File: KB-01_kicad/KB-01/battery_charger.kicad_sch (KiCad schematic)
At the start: 37 parts, among them IC1 MAX17048G+T10, J12 Conn_01x01_Socket, J3 USB_C_Receptacle_USB2.0_14P, J4 Conn_01x02_Socket, J5 Conn_01x01_Socket, SW2 Power button, U1 BQ25895, U2 TS3USB30ERSWR, U3 TLV70430DBVR

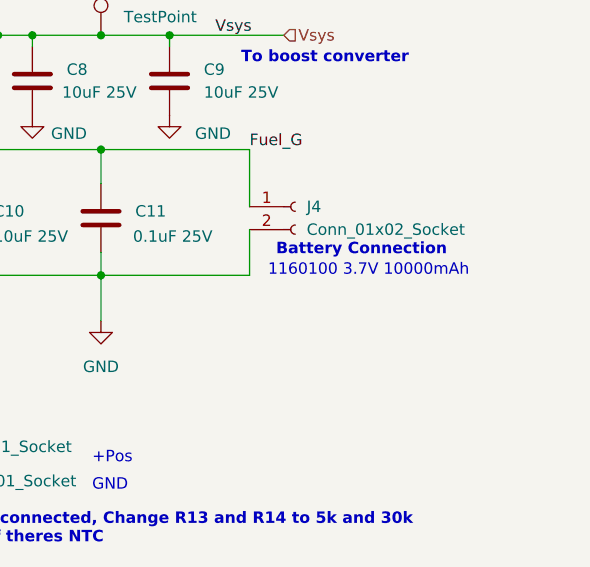
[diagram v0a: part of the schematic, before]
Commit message: all
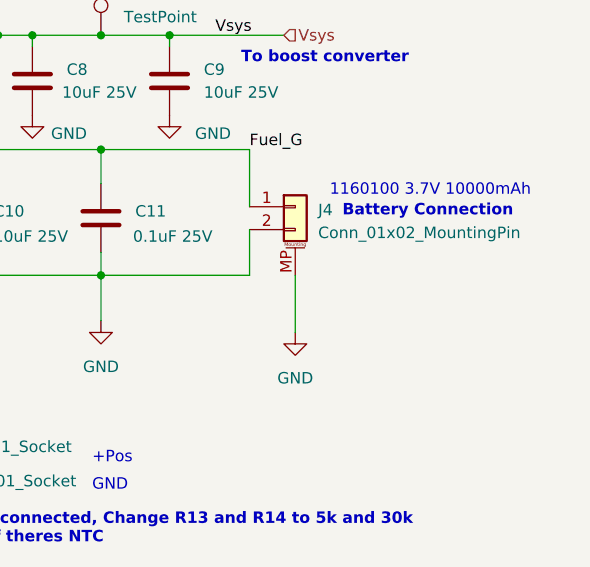
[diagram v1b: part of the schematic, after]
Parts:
- J4: value Conn_01x02_Socket -> Conn_01x02_MountingPin; footprint Connector_JST:JST_PH_B2B-PH-SM4-TB_1x02-1MP_P2.00mm_Vertical -> (none); symbol Connector:Conn_01x02_Socket -> Connector_Generic_MountingPin:Conn_01x02_MountingPin; mouser 306-B2BPHSM4TBLFSN -> (none)
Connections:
- net GND: now also J4.MP (MountPin)
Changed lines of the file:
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@@
 	(text " 1160100 3.7V 10000mAh"
 		(exclude_from_sim no)
-		(at 272.034 84.582 0)
+		(at 278.892 75.692 0)
 		(effects
 			(font
@@
 	(text "Battery Connection"
 		(exclude_from_sim no)
-		(at 271.526 82.296 0)
+		(at 278.892 77.978 0)
 		(effects
 			(font
@@
 	(wire
 		(pts
+			(xy 264.16 85.09) (xy 264.16 91.44)
+		)
+		(stroke
+			(width 0)
+			(type default)
+		)
+	)
+	(wire
+		(pts
 			(xy 62.23 58.42) (xy 64.77 58.42)
 		)
@@
 	)
 	(symbol
+		(lib_id "power:GND")
+		(at 264.16 91.44 0)
+		(unit 1)
+		(body_style 1)
+		(exclude_from_sim no)
+		(in_bom yes)
+		(on_board yes)
+		(in_pos_files yes)
+		(dnp no)
+		(fields_autoplaced yes)
+		(property "Reference" "#PWR089"
+			(at 264.16 97.79 0)
+			(hide yes)
+			(show_name no)
+			(do_not_autoplace no)
+			(effects
+				(font
+					(size 1.27 1.27)
+				)
+			)
+		)
+		(property "Value" "GND"
+			(at 264.16 96.52 0)
+			(show_name no)
+			(do_not_autoplace no)
+			(effects
+				(font
+					(size 1.27 1.27)
+				)
+			)
+		)
+		(property "Footprint" ""
+			(at 264.16 91.44 0)
+			(hide yes)
+			(show_name no)
+			(do_not_autoplace no)
+			(effects
+				(font
+					(size 1.27 1.27)
+				)
+			)
+		)
+		(property "Datasheet" ""
+			(at 264.16 91.44 0)
+			(hide yes)
+			(show_name no)
+			(do_not_autoplace no)
+			(effects
+				(font
+					(size 1.27 1.27)
+				)
+			)
+		)
+		(property "Description" "Power symbol creates a global label with name \"GND\" , ground"
+			(at 264.16 91.44 0)
+			(hide yes)
+			(show_name no)
+			(do_not_autoplace no)
+			(effects
+				(font
+					(size 1.27 1.27)
+				)
+			)
+		)
+		(pin "1"
+		)
+		(instances
+			(project "KB-01"
+				(path "/e6144e29-1dc4-45a8-93e7-988a20131b94/8a655b9b-8849-4070-bc16-b30b70cfa2c5"
+					(reference "#PWR089")
+					(unit 1)
+				)
+			)
+		)
+	)
+	(symbol
 		(lib_id "Device:R")
 		(at 151.13 96.52 0)
@@
 	)
 	(symbol
-		(lib_id "Connector:Conn_01x02_Socket")
+		(lib_id "Connector_Generic_MountingPin:Conn_01x02_MountingPin")
 		(at 264.16 77.47 0)
 		(unit 1)
@@
 		(fields_autoplaced yes)
 		(property "Reference" "J4"
-			(at 265.43 77.4699 0)
+			(at 266.7 77.8255 0)
 			(show_name no)
 			(do_not_autoplace no)
@@
 			)
 		)
-		(property "Value" "Conn_01x02_Socket"
-			(at 265.43 80.0099 0)
+		(property "Value" "Conn_01x02_MountingPin"
+			(at 266.7 80.3655 0)
 			(show_name no)
 			(do_not_autoplace no)
@@
 			)
 		)
-		(property "Footprint" "Connector_JST:JST_PH_B2B-PH-SM4-TB_1x02-1MP_P2.00mm_Vertical"
+		(property "Footprint" ""
 			(at 264.16 77.47 0)
 			(hide yes)
@@
 			)
 		)
-		(property "Description" "Generic connector, single row, 01x02, script generated"
-			(at 264.16 77.47 0)
-			(hide yes)
-			(show_name no)
-			(do_not_autoplace no)
-			(effects
-				(font
-					(size 1.27 1.27)
-				)
-			)
-		)
-		(property "mouser" "306-B2BPHSM4TBLFSN"
-			(at 264.16 77.47 0)
-			(hide yes)
-			(show_name no)
-			(do_not_autoplace no)
-			(effects
-				(font
-					(size 1.27 1.27)
-				)
-			)
-		)
-		(property "SNAPEDA_PN" ""
+		(property "Description" "Generic connectable mounting pin connector, single row, 01x02, script generated (kicad-library-utils/schlib/autogen/connector/)"
 			(at 264.16 77.47 0)
 			(hide yes)
@@
 		(pin "2"
 		)
+		(pin "MP"
+		)
 		(instances

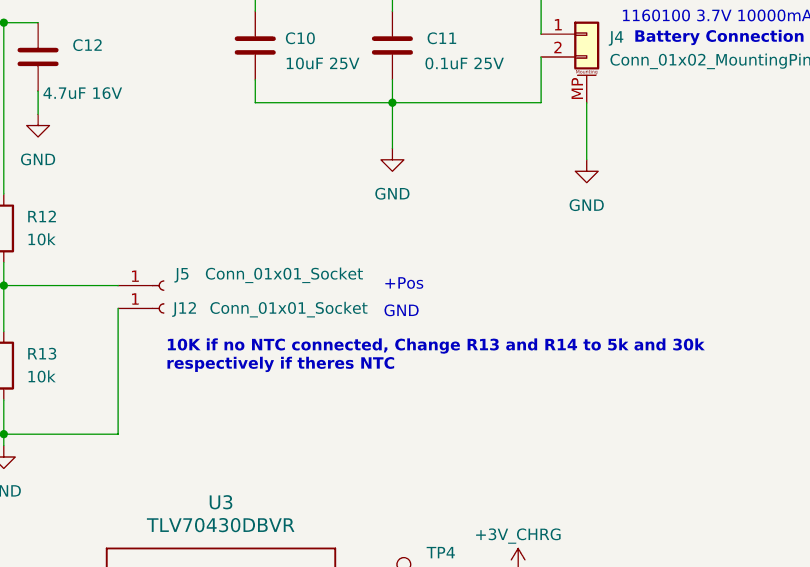
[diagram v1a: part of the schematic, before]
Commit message: all
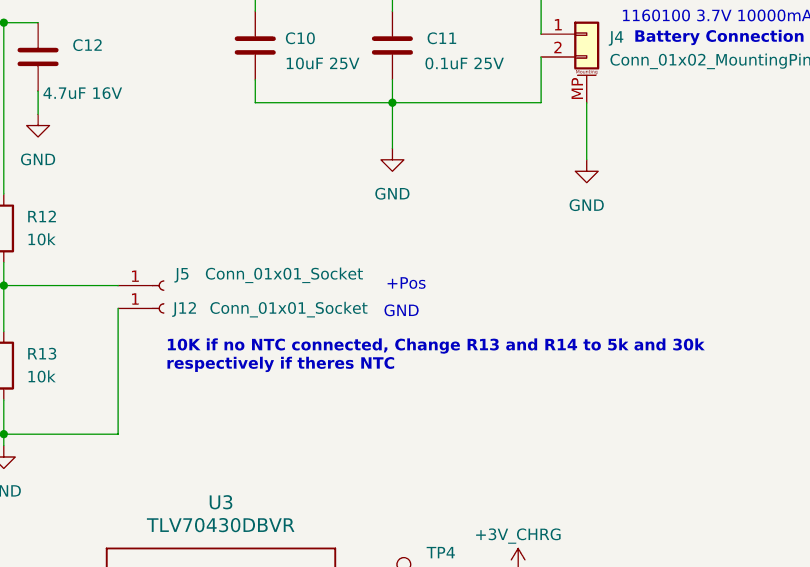
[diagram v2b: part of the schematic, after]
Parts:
- J4: footprint (none) -> Connector_JST:JST_PH_S2B-PH-SM4-TB_1x02-1MP_P2.00mm_Horizontal; mouser (none) -> 306-S2BPHSM4TBLFSN
- U3: footprint DBV0005A_N -> TLV70430DBVR:DBV0005A_M
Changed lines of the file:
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@@
 	(text "+Pos\n"
 		(exclude_from_sim no)
-		(at 243.84 105.41 0)
+		(at 244.094 105.41 0)
 		(effects
 			(font
@@
 			)
 		)
-		(property "Footprint" "DBV0005A_N"
+		(property "Footprint" "TLV70430DBVR:DBV0005A_M"
 			(at 223.52 144.78 0)
 			(hide yes)
@@
 			)
 		)
-		(property "Footprint" ""
+		(property "Footprint" "Connector_JST:JST_PH_S2B-PH-SM4-TB_1x02-1MP_P2.00mm_Horizontal"
 			(at 264.16 77.47 0)
 			(hide yes)
@@
 			(at 264.16 77.47 0)
 			(hide yes)
+			(show_name no)
+			(do_not_autoplace no)
+			(effects
+				(font
+					(size 1.27 1.27)
+				)
+			)
+		)
+		(property "mouser" "306-S2BPHSM4TBLFSN  "
+			(at 264.16 77.47 0)
+			(hide yes)
